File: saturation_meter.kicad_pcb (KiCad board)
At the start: 2 copper layers, 138 x 111 mm, 64 parts, among them J1 Vin, J2 DUT, J3 Inputs, J4 Outputs, J5 UC, Q1 BUK556, Q2 BUK556, Q3 BC328, U1 LF33_TO220, U2 IR2112

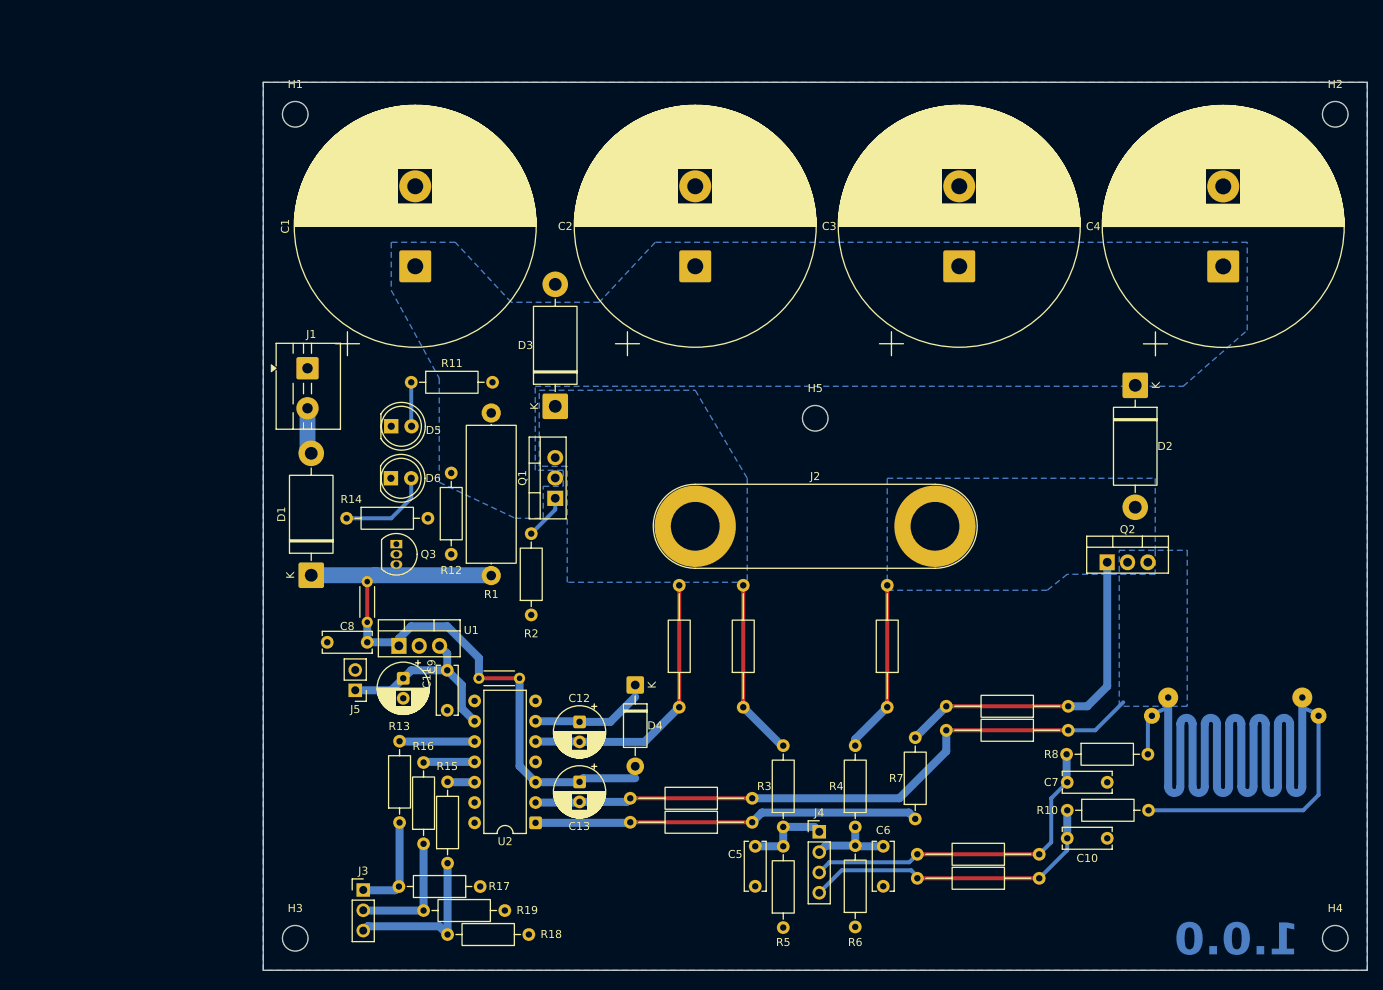
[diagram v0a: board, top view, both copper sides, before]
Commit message: Added pictures and updated design sheet
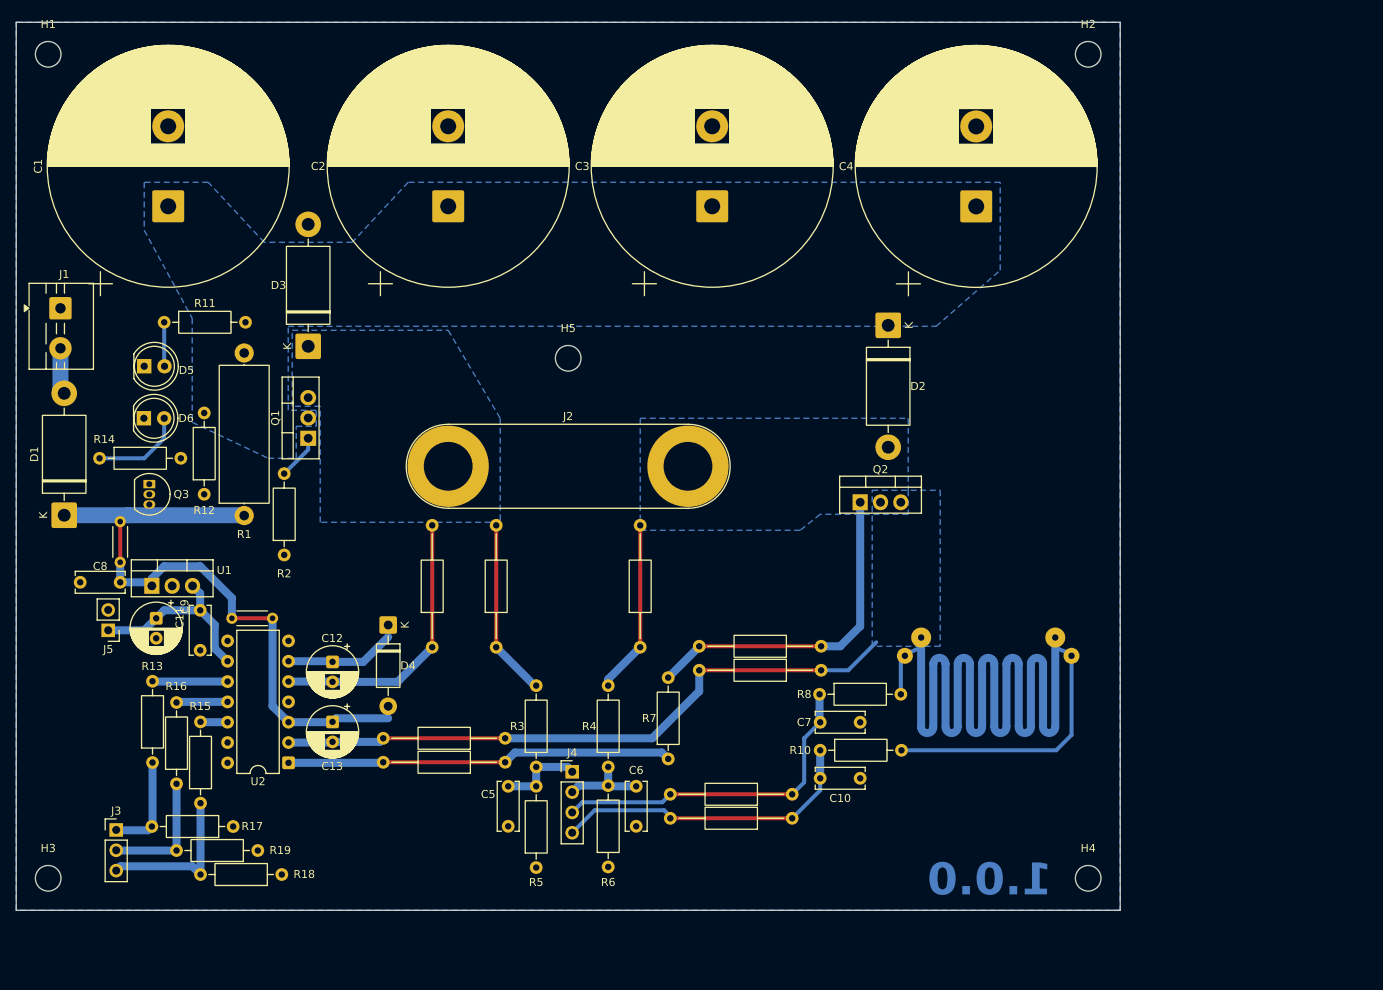
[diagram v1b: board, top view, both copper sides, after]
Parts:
- moved R13 31.8 mm to (95.7, 130.5)
- moved R17 31.8 mm to (105.7, 138.5)
- moved C1 31.8 mm to (97.6, 61.0)
- moved C10 31.8 mm to (179.1, 132.5)
- moved C11 31.8 mm to (101.6, 111.5)
- moved C12 31.8 mm to (118.2, 118.0)
- moved C2 31.8 mm to (132.6, 61.0)
- moved C3 31.8 mm to (165.6, 61.0)
- moved C5 31.8 mm to (140.1, 133.5)
- moved C6 31.8 mm to (156.1, 133.5)
- moved C7 31.8 mm to (179.1, 125.5)
- moved C8 31.8 mm to (91.6, 108.0)
- moved C9 31.8 mm to (96.1, 112.5)
- moved D1 31.8 mm to (84.6, 99.6)
- moved D2 31.8 mm to (187.6, 75.9)
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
